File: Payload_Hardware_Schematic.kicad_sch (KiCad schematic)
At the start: 3 parts, among them U1 STM32F411 BlackPill, U2 MPM3610, U3 MPM3610

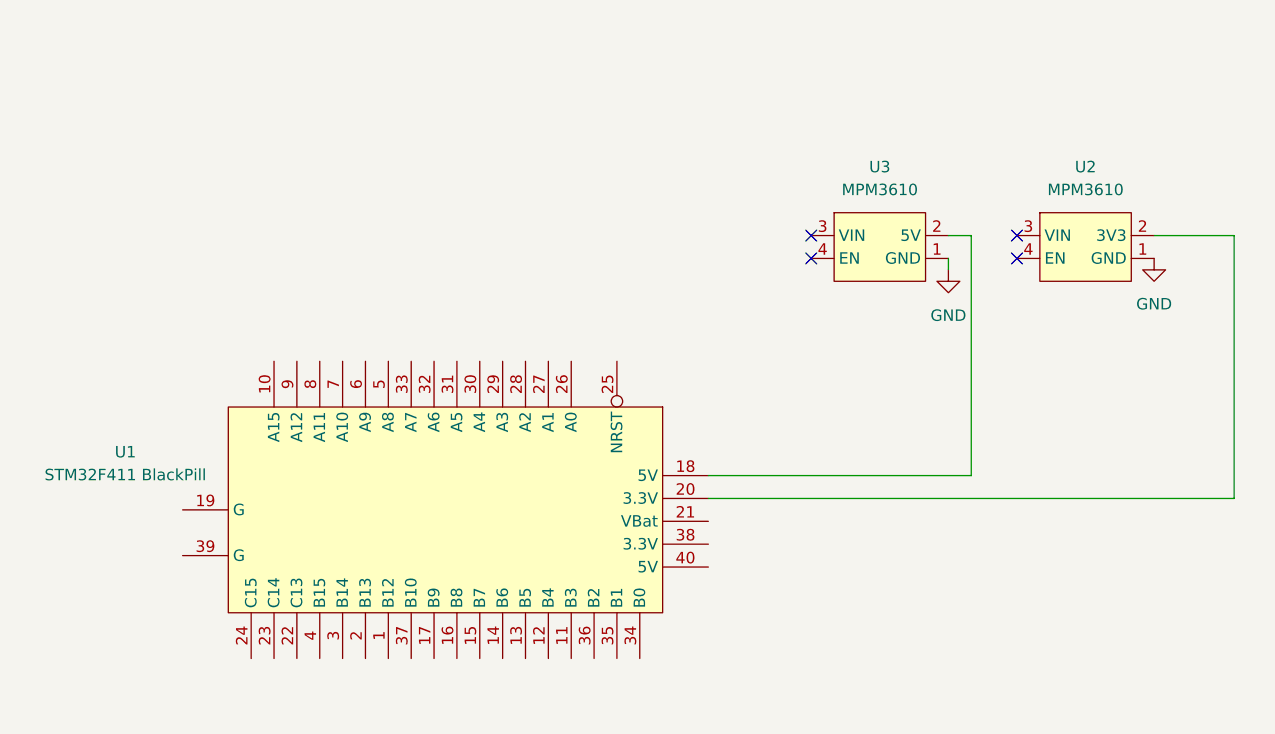
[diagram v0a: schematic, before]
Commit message: added pins
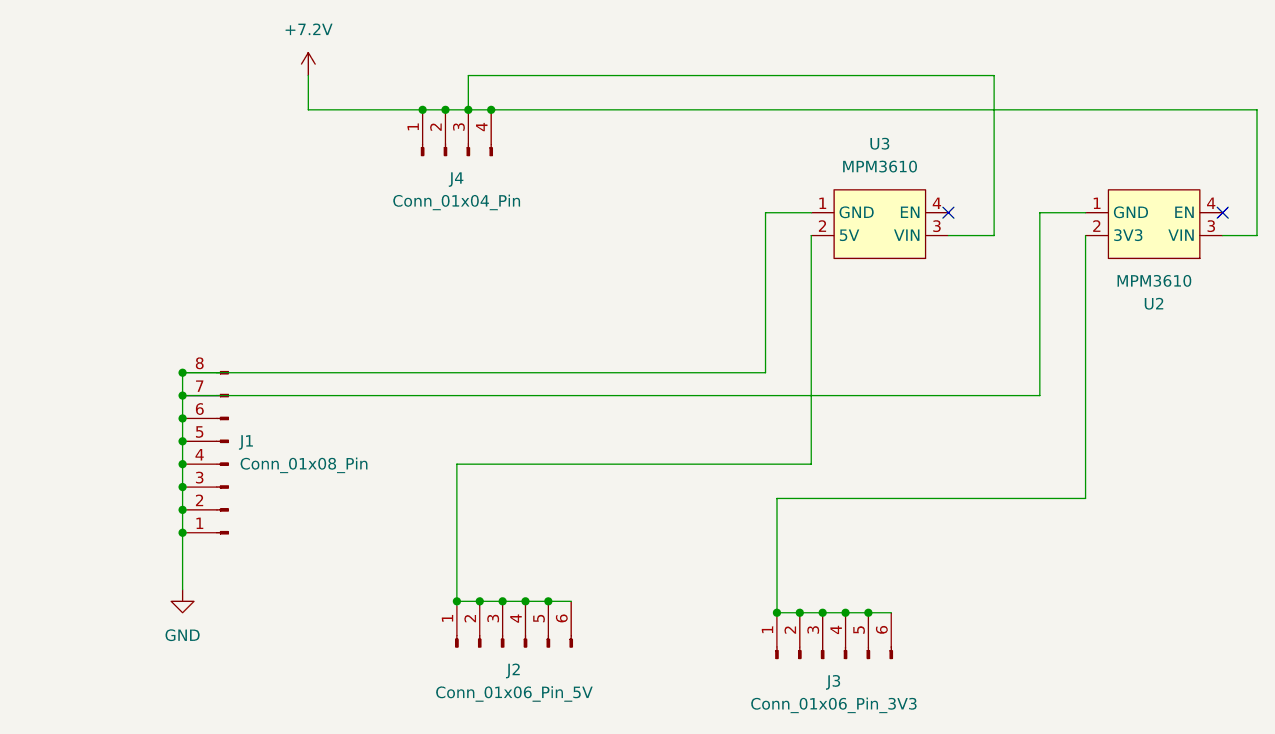
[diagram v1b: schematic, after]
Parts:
- removed U1: STM32F411 BlackPill, Payload-STM32:STM32F411_Black_Pill, symbol Payload-STM32:STM32F411_Black_Pill
- added J1: Conn_01x08_Pin, symbol Connector:Conn_01x08_Pin
- added J2: Conn_01x06_Pin_5V, symbol Connector:Conn_01x06_Pin
- added J3: Conn_01x06_Pin_3V3, symbol Connector:Conn_01x06_Pin
- added J4: Conn_01x04_Pin, symbol Connector:Conn_01x04_Pin
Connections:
- net GND: now also J1.1 (Pin_1), J1.2 (Pin_2), J1.3 (Pin_3), J1.4 (Pin_4), J1.5 (Pin_5), J1.6 (Pin_6), J1.7 (Pin_7), J1.8 (Pin_8)
- net at U3.2 (5V): now also J2.1 (Pin_1), J2.2 (Pin_2), J2.3 (Pin_3), J2.4 (Pin_4), J2.5 (Pin_5), J2.6 (Pin_6)
- net +7.2V: now reaches U3.3 (VIN)
- net +7.2V: now also U2.3 (VIN), J4.1 (Pin_1), J4.2 (Pin_2), J4.3 (Pin_3), J4.4 (Pin_4)
- net at U2.2 (3V3): now also J3.1 (Pin_1), J3.2 (Pin_2), J3.3 (Pin_3), J3.4 (Pin_4), J3.5 (Pin_5), J3.6 (Pin_6)
- no-connect marks 4 -> 2
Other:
- moved on the sheet: U2, U3
